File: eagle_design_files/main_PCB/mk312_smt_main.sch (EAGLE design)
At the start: 137 parts, among them IC1 MEGA16-A, J11 Z-S311024S1GK1A, J2 REMOTE INPUT, J3 LINK INPUT, J4 MIC INPUT, J5 LINE INPUT, J6 OUTPUT A, J7 OUTPUT B, J8 VDC INPUT, J9 X6511FV-06-C85D32, Q1 N-HEXFET-2D_SOT232-IRLL2705, Q2 N-HEXFET-2D_SOT232-IRLL2705, Q3 BSP170PH6327, Q4 N-HEXFET-2D_SOT232-IRLL2705, Q5 N-HEXFET-2D_SOT232-IRLL2705, Q6 BSP170PH6327, U10 LM358DR2G, U2 LM324DT, U4 LM358DR2G, U9 MAX232ESE+T, Y2 8MHZ

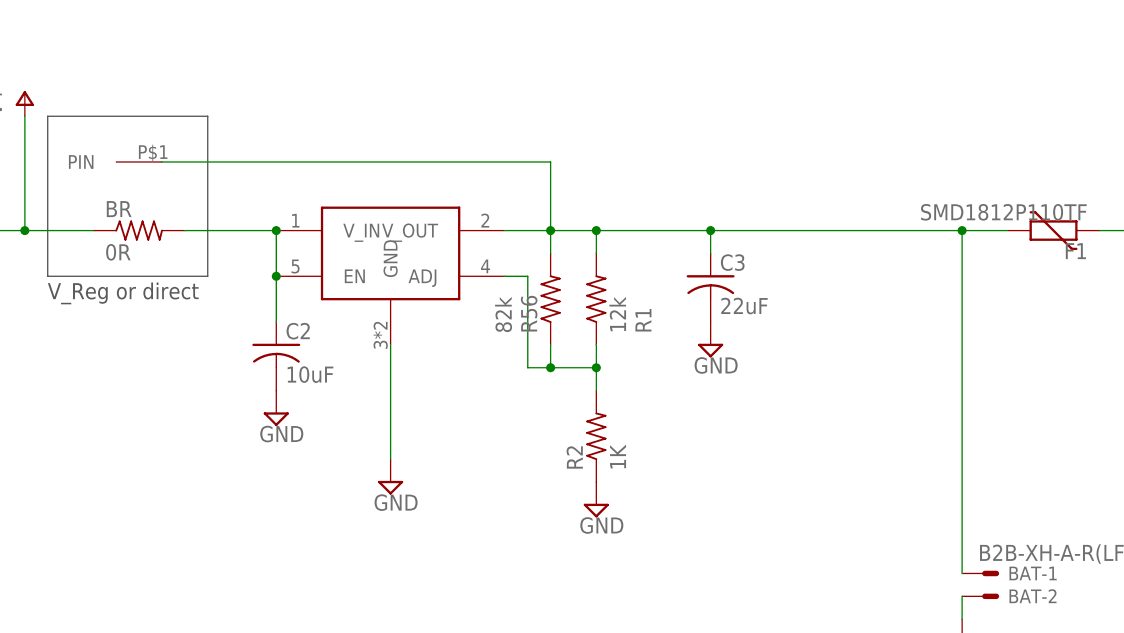
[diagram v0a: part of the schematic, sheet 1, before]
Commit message: Add files via upload
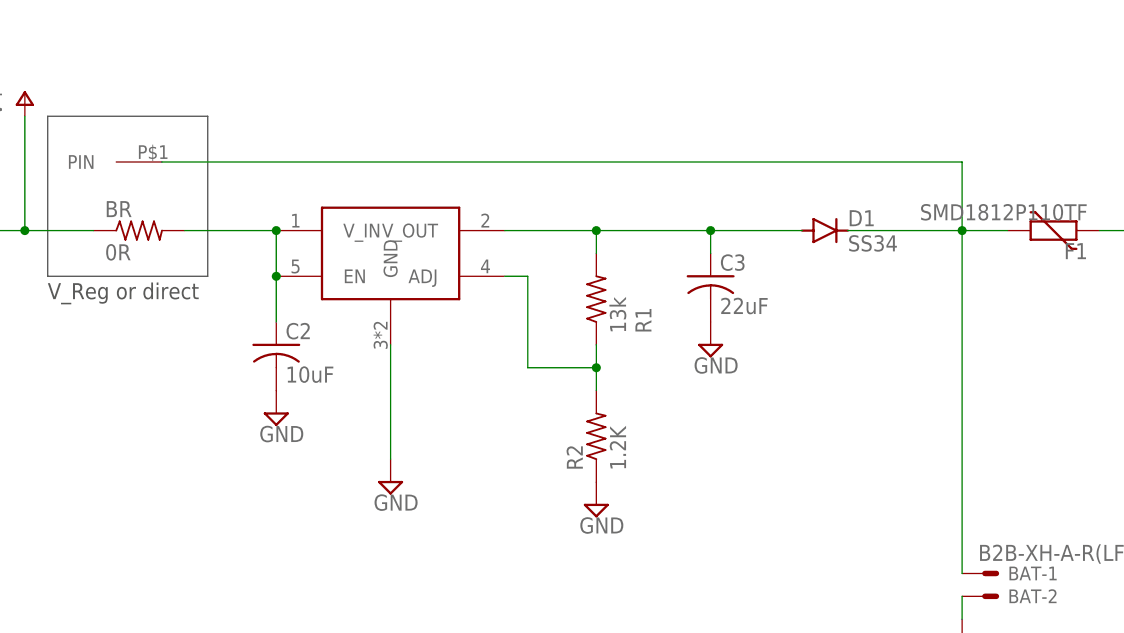
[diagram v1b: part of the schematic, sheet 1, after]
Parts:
- removed R56: 82k, rcl:R-US_R0805
- added D1: SS34, diode:S1M
- R1: value 12k -> 13k
- R2: value 1K -> 1.2K
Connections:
- new net N$11: C3.1, D1.A, R1.2, V_REG.V_OUT
- net N$43: no longer R56.1
- net VM_OUT: now also D1.C; no longer C3.1, R1.2, R56.2, V_REG.V_OUT
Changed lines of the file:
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@@
 <part name="R42" library="rcl" deviceset="R-US_" device="R0805" value="100K"/>
 <part name="J8" library="SparkFun-Connectors" deviceset="POWER_JACK" device="SLT" value="VDC INPUT"/>
-<part name="R1" library="rcl" deviceset="R-US_" device="R0805" value="12k"/>
-<part name="R2" library="rcl" deviceset="R-US_" device="R0805" value="1K"/>
+<part name="R1" library="rcl" deviceset="R-US_" device="R0805" value="13k"/>
+<part name="R2" library="rcl" deviceset="R-US_" device="R0805" value="1.2K"/>
 <part name="GND20" library="supply2" deviceset="GND" device=""/>
 <part name="GND23" library="supply2" deviceset="GND" device=""/>
@@
 <part name="TU" library="jumper" library_urn="urn:adsk.eagle:library:252" deviceset="SJ" device="" package3d_urn="urn:adsk.eagle:package:15471/1" value="0"/>
 <part name="V_REG" library="MK312parts" deviceset="TPS73801" device="SOT223-6" package3d_urn="urn:adsk.eagle:package:42943783/1"/>
-<part name="R56" library="rcl" deviceset="R-US_" device="R0805" value="82k"/>
 <part name="Q1" library="MK312parts" deviceset="N-HEXFET-2D_?-*" device="SOT232" package3d_urn="urn:adsk.eagle:package:29522/2" technology="IRLL2705"/>
 <part name="Q2" library="MK312parts" deviceset="N-HEXFET-2D_?-*" device="SOT232" package3d_urn="urn:adsk.eagle:package:29522/2" technology="IRLL2705"/>
@@
 <part name="BR" library="rcl" library_urn="urn:adsk.eagle:library:334" deviceset="R-US_" device="R0805" package3d_urn="urn:adsk.eagle:package:23553/2" value="0R"/>
 <part name="U$2" library="MK312parts" deviceset="PAD_0805" device=""/>
+<part name="D1" library="diode" library_urn="urn:adsk.eagle:library:210" deviceset="S1M" device="" package3d_urn="urn:adsk.eagle:package:43460/3" value="SS34"/>
 </parts>
 <sheets>
@@
 </instance>
 <instance part="V_REG" gate="G$1" x="86.36" y="142.24" smashed="yes"/>
-<instance part="R56" gate="G$1" x="104.14" y="137.16" smashed="yes" rot="R90">
-<attribute name="NAME" x="102.6414" y="133.35" size="1.778" layer="95" rot="R90"/>
-<attribute name="VALUE" x="99.822" y="133.35" size="1.778" layer="96" rot="R90"/>
-</instance>
 <instance part="BR" gate="G$1" x="58.42" y="144.78" smashed="yes">
 <attribute name="NAME" x="54.61" y="146.2786" size="1.778" layer="95"/>
@@
 </instance>
 <instance part="U$2" gate="G$1" x="60.96" y="152.4" smashed="yes" rot="R180"/>
+<instance part="D1" gate="G$1" x="134.62" y="144.78" smashed="yes">
+<attribute name="NAME" x="137.16" y="145.2626" size="1.778" layer="95"/>
+<attribute name="VALUE" x="137.16" y="142.4686" size="1.778" layer="96"/>
+</instance>
 </instances>
 <busses>
@@
 <wire x1="109.22" y1="129.54" x2="109.22" y2="127" width="0.1524" layer="91"/>
 <wire x1="101.6" y1="139.7" x2="101.6" y2="129.54" width="0.1524" layer="91"/>
-<wire x1="101.6" y1="129.54" x2="104.14" y2="129.54" width="0.1524" layer="91"/>
 <junction x="109.22" y="129.54"/>
-<wire x1="104.14" y1="129.54" x2="109.22" y2="129.54" width="0.1524" layer="91"/>
-<pinref part="R56" gate="G$1" pin="1"/>
+<wire x1="101.6" y1="129.54" x2="109.22" y2="129.54" width="0.1524" layer="91"/>
 <wire x1="99.06" y1="139.7" x2="101.6" y2="139.7" width="0.1524" layer="91"/>
-<wire x1="104.14" y1="132.08" x2="104.14" y2="129.54" width="0.1524" layer="91"/>
-<junction x="104.14" y="129.54"/>
 <pinref part="V_REG" gate="G$1" pin="ADJ"/>
 </segment>
@@
 <net name="VM_OUT" class="2">
 <segment>
-<pinref part="R1" gate="G$1" pin="2"/>
-<wire x1="109.22" y1="144.78" x2="109.22" y2="142.24" width="0.1524" layer="91"/>
-<wire x1="109.22" y1="144.78" x2="121.92" y2="144.78" width="0.1524" layer="91"/>
-<wire x1="121.92" y1="144.78" x2="149.86" y2="144.78" width="0.1524" layer="91"/>
-<pinref part="C3" gate="G$1" pin="1"/>
+<pinref part="U$2" gate="G$1" pin="PIN"/>
+<pinref part="F1" gate="G$1" pin="1"/>
 <wire x1="149.86" y1="144.78" x2="154.94" y2="144.78" width="0.1524" layer="91"/>
-<wire x1="121.92" y1="142.24" x2="121.92" y2="144.78" width="0.1524" layer="91"/>
-<junction x="121.92" y="144.78"/>
-<junction x="109.22" y="144.78"/>
-<wire x1="99.06" y1="144.78" x2="104.14" y2="144.78" width="0.1524" layer="91"/>
-<wire x1="104.14" y1="144.78" x2="109.22" y2="144.78" width="0.1524" layer="91"/>
-<pinref part="R56" gate="G$1" pin="2"/>
-<wire x1="104.14" y1="142.24" x2="104.14" y2="144.78" width="0.1524" layer="91"/>
-<junction x="104.14" y="144.78"/>
-<pinref part="V_REG" gate="G$1" pin="V_OUT"/>
-<wire x1="60.96" y1="152.4" x2="104.14" y2="152.4" width="0.1524" layer="91"/>
-<wire x1="104.14" y1="152.4" x2="104.14" y2="144.78" width="0.1524" layer="91"/>
-<pinref part="F1" gate="G$1" pin="1"/>
 <pinref part="BAT" gate="-1" pin="S"/>
 <wire x1="149.86" y1="106.68" x2="149.86" y2="144.78" width="0.1524" layer="91"/>
+<pinref part="D1" gate="G$1" pin="C"/>
+<wire x1="137.16" y1="144.78" x2="149.86" y2="144.78" width="0.1524" layer="91"/>
 <junction x="149.86" y="144.78"/>
-<pinref part="U$2" gate="G$1" pin="PIN"/>
+<wire x1="60.96" y1="152.4" x2="149.86" y2="152.4" width="0.1524" layer="91"/>
+<wire x1="149.86" y1="152.4" x2="149.86" y2="144.78" width="0.1524" layer="91"/>
 </segment>
 </net>
@@
 </segment>
 </net>
+<net name="N$11" class="2">
+<segment>
+<pinref part="C3" gate="G$1" pin="1"/>
+<wire x1="121.92" y1="142.24" x2="121.92" y2="144.78" width="0.1524" layer="91"/>
+<pinref part="R1" gate="G$1" pin="2"/>
+<wire x1="109.22" y1="144.78" x2="109.22" y2="142.24" width="0.1524" layer="91"/>
+<wire x1="109.22" y1="144.78" x2="121.92" y2="144.78" width="0.1524" layer="91"/>
+<junction x="109.22" y="144.78"/>
+<pinref part="V_REG" gate="G$1" pin="V_OUT"/>
+<wire x1="99.06" y1="144.78" x2="109.22" y2="144.78" width="0.1524" layer="91"/>
+<pinref part="D1" gate="G$1" pin="A"/>
+<wire x1="121.92" y1="144.78" x2="132.08" y2="144.78" width="0.1524" layer="91"/>
+<junction x="121.92" y="144.78"/>
+</segment>
+</net>
